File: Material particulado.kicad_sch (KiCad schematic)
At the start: 10 parts, among them U1 ESP32-S3-WROOM-1, U2 LM35-D, U3 LM358_DFN, U4 LM358_DFN

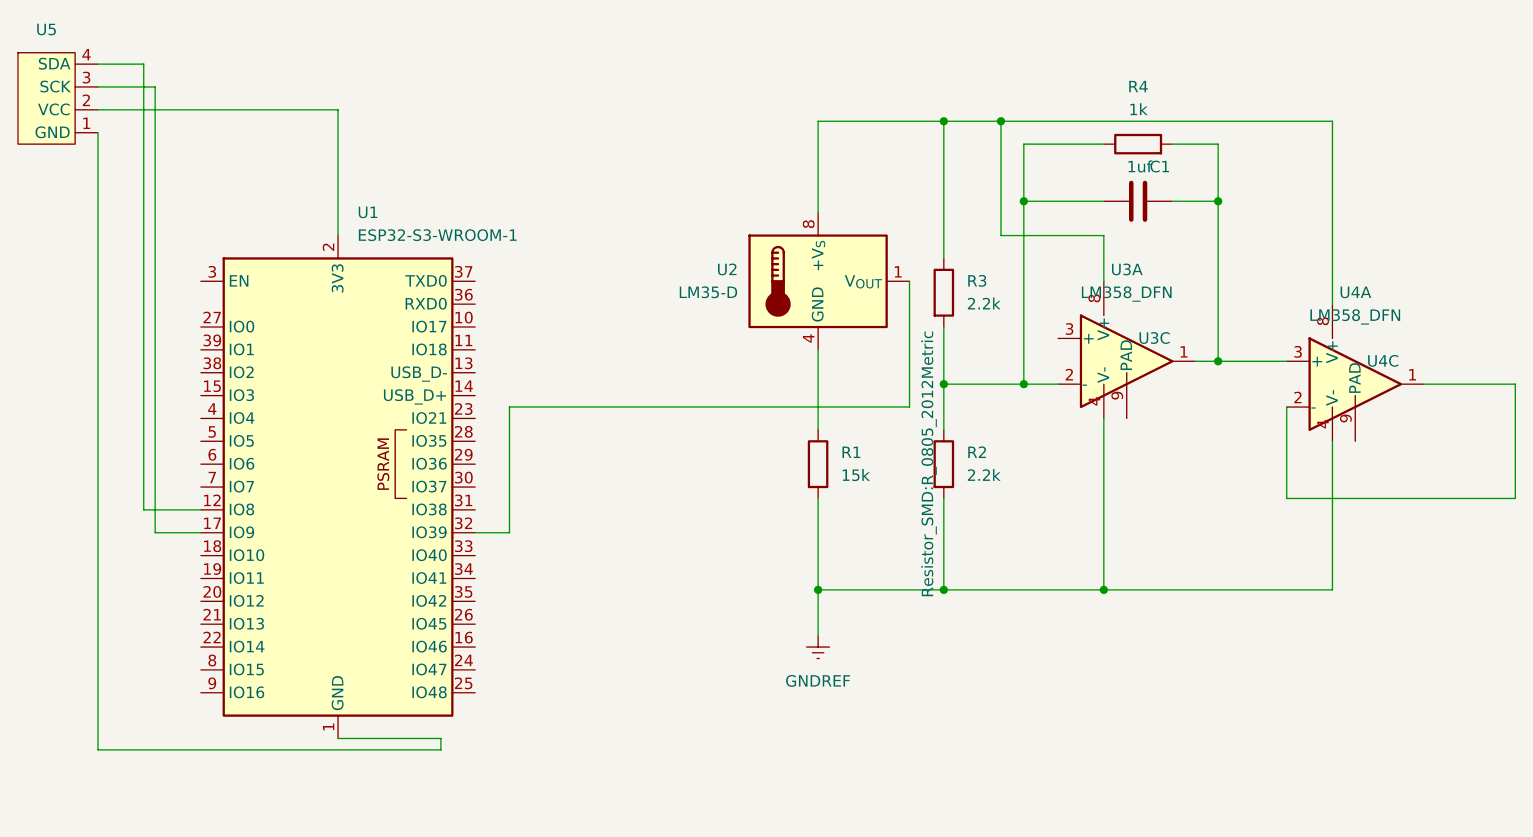
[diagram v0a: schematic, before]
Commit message: Puse etiquetas y corte cables
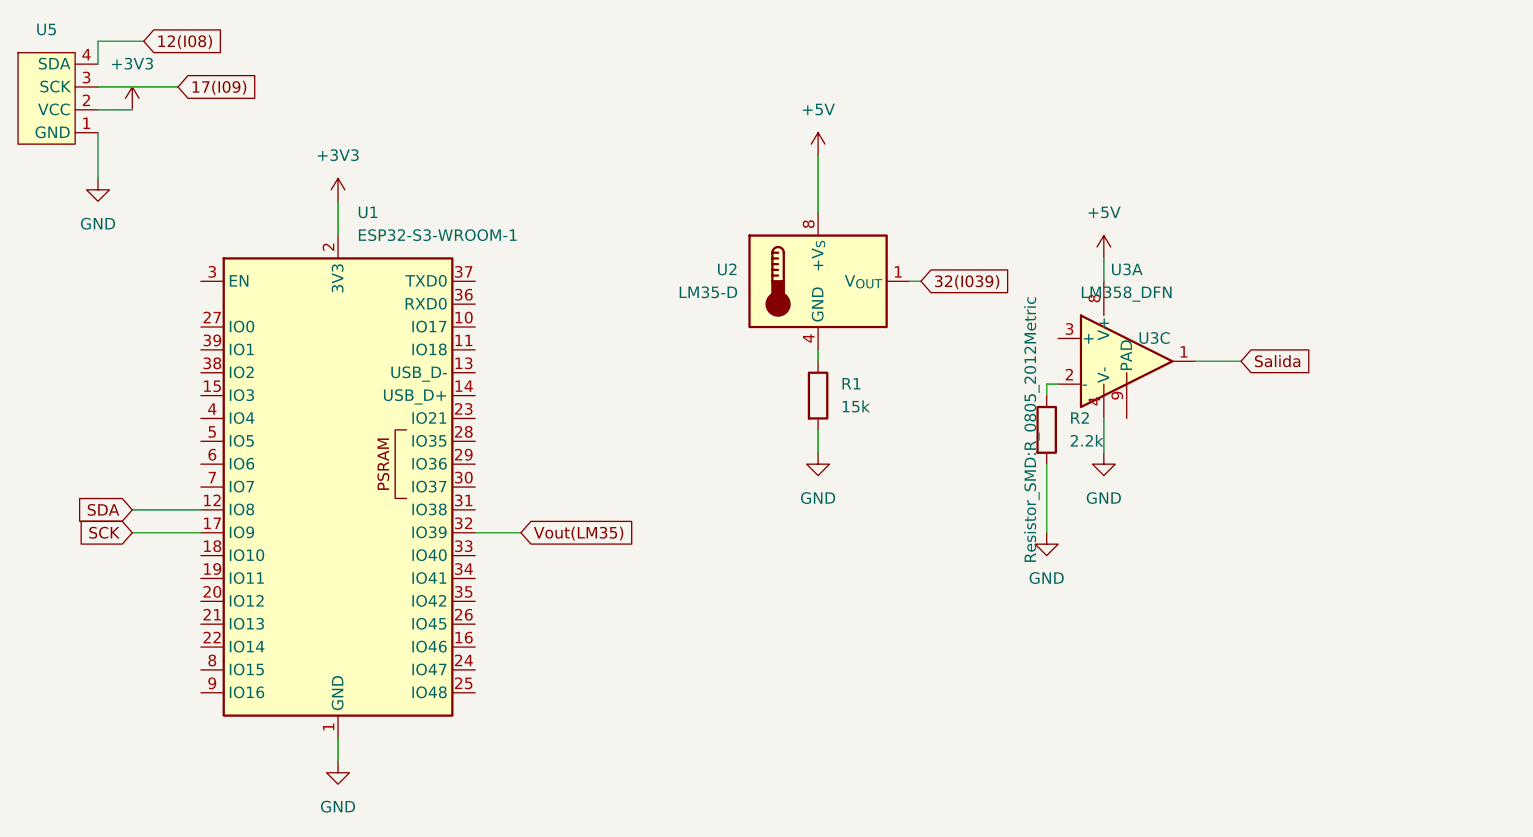
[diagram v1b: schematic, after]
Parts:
- removed C1: 1uf, Capacitor_SMD:C_0805_2012Metric, symbol Device:C
- removed R3: 2.2k, Resistor_SMD:R_0805_2012Metric, symbol Device:R
- removed R4: 1k, Resistor_SMD:R_0805_2012Metric_Pad1.20x1.40mm_HandSolder, symbol Device:R
- removed U4: LM358_DFN, Package_DFN_QFN:DFN-8-1EP_2x2mm_P0.5mm_EP1.05x1.75mm, symbol Amplifier_Operational:LM358_DFN
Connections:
- net GNDREF is gone; now on net GND: R1.2, R2.2, U3.4 (V-)
- net +5V: now reaches U2.8 (+V_{S}), U3.8 (V+)
- net Salida: now reaches U3.1
- net GND: now reaches U1.1 (GND), U1.40 (GND), U1.41 (GND), U5.1 (GND)
- net +3V3: now reaches U1.2 (3V3), U5.2 (VCC)
- net 17(I09): now reaches U5.3 (SCK)
- net 17(I09): no longer U1.17 (IO9)
- net 12(I08): now reaches U5.4 (SDA)
- net 12(I08): no longer U1.12 (IO8)
- net 32(I039): now reaches U2.1 (V_{OUT})
- net 32(I039): no longer U1.32 (IO39)
- new net SCK: U1.17 (IO9)
- new net SDA: U1.12 (IO8)
- new net Vout(LM35): U1.32 (IO39)
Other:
- moved on the sheet: R1, R2
